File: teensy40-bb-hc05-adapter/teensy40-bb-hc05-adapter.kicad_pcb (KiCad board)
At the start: 2 copper layers, 18 x 71.6 mm, 17 parts, among them J1 Conn_01x06_0.1_Header, J2 Conn_01x06_0.1_Socket, J3 Conn_01x08, J4 Conn_01x08, U1 74LVC1G17, U2 74LVC1G14, U3 Teensy4.0_WithBottomAndEdge

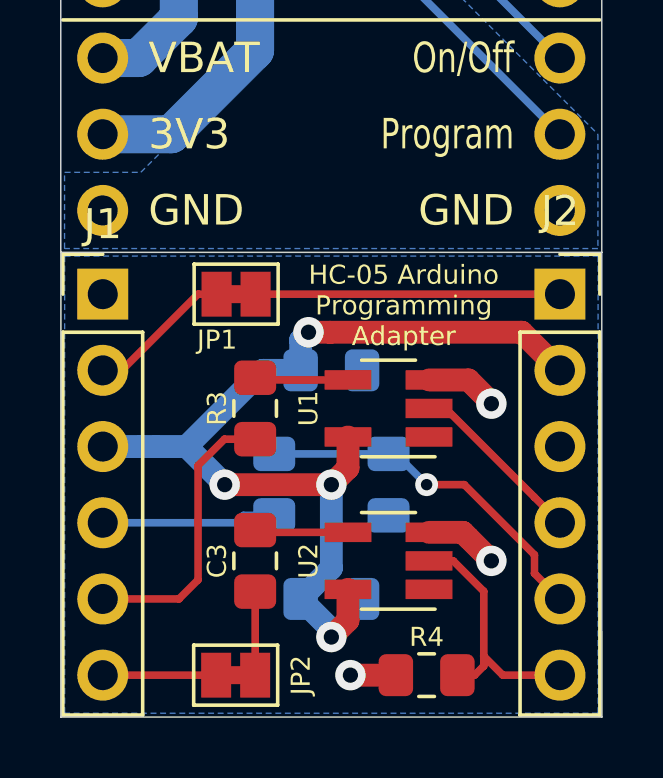
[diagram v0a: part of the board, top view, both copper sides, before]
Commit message: Clean up positions
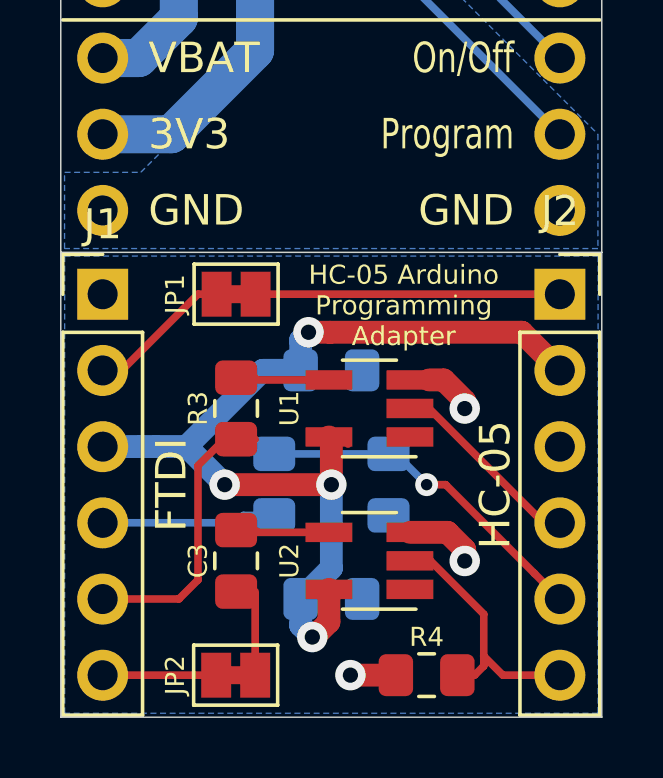
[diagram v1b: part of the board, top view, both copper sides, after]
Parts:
- moved U1 0.64 mm to (135.9, 136.1)
- moved U2 0.64 mm to (135.9, 141.2)
- moved C3 0.63 mm to (131.4, 141.2)
- moved R3 0.63 mm to (131.4, 136.1)
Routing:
- net Net-(R3-Pad2): track 3.13 -> 4.40 mm
- net GND: track 6.41 -> 5.69 mm
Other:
- board text added: "RXI"
- board text added: "RXO"
- board text added: "TXI"
- board text added: "TXO"
- board text removed: "RX"
- board text removed: "TX"
